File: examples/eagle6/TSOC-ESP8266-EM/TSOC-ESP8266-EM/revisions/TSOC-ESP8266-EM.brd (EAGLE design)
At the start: 38.1 x 25.4 mm, 21 parts, among them Q1 MMBT2222A, U1 ESP8266-12-12W

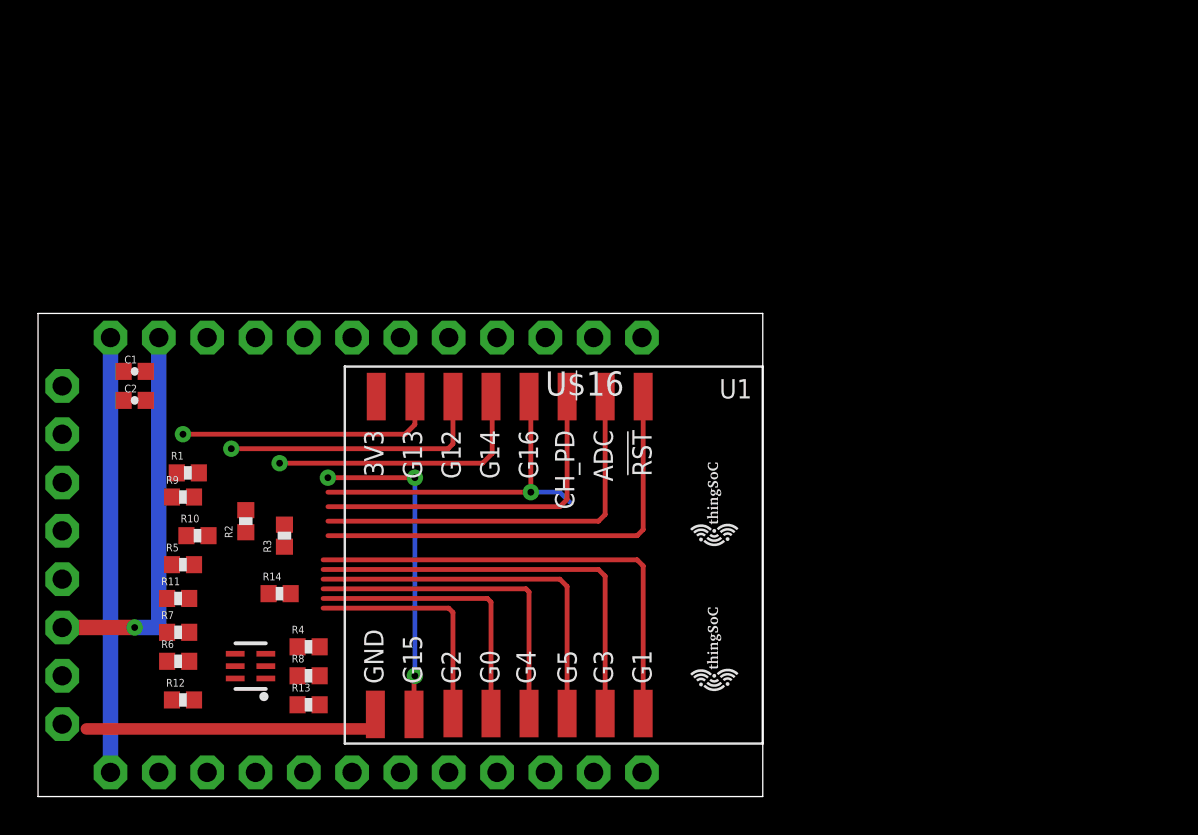
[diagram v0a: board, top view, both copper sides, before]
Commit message: update modules
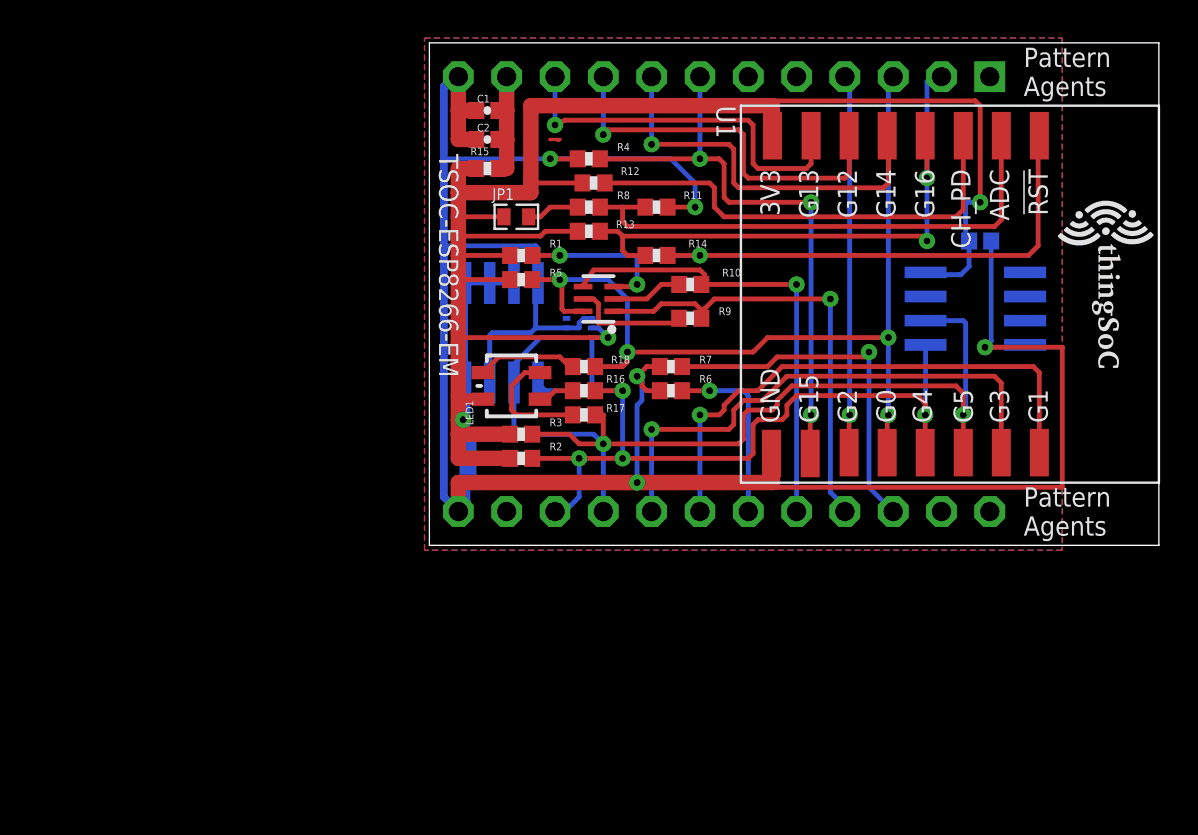
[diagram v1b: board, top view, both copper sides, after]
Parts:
- removed U$16: TSOC-32-BB, thingSoC:TSOC-BB-S32
- added C3, C4: 0.1uF, PatternAgents-ProtoPads:0402-CAP
- added JP1: (no value), PatternAgents-ProtoPads:JMP-2-NO-0402
- added LED1: LED-TRICOLOR, SparkFun-LED:LED-TRICOLOR-SMD
- added R15: 0.01, PatternAgents-ProtoPads:0402-RES
- added R16, R17, R18: 560, PatternAgents-ProtoPads:0402-RES
- added TSOC: TSOC-24-BB, thingSoC:TSOC-BB-S24
- added U$11: PA_LOGO_SYMMED, PatternAgents-Logos:PA_LOGO_AGENT_MED_SYM
- added U2: EEPROM-I2CSMD, SparkFun-DigitalIC:SO08
- added U3: TMP102, SparkFun-Sensors:SOT563
- added U4: ATECC108, SparkFun-DigitalIC:SOIC8
- U$19, U$20: value TSOC-LOGO-SMALL -> TSOC-LOGO-MED; device thingSoC:TSOC-LOGO-SML -> thingSoC:TSOC-LOGO-MED
- moved R12 34.7 mm to (8.89, 19.6), turned to 180 degrees
- moved R11 32.5 mm to (12.2, 18.3)
- moved U$20 31.1 mm to (35.8, 17.0), turned to 270 degrees
- moved R4 29.6 mm to (8.64, 20.8)
- moved R6 29.6 mm to (13.0, 8.64)
- moved R7 29.4 mm to (13.0, 9.91)
- moved R10 29.1 mm to (14.0, 14.2), turned to 180 degrees
- moved R13 28.9 mm to (8.64, 17.0), turned to 180 degrees
- moved R8 28.7 mm to (8.64, 18.3), turned to 180 degrees
- moved R9 28.3 mm to (14.0, 12.4), turned to 180 degrees
- moved R14 26.6 mm to (12.2, 15.7)
- moved Q1 26.6 mm to (9.14, 13.5)
- moved U1 24.9 mm to (27.2, 13.5)
- moved R5 23.3 mm to (5.08, 14.5), turned to 180 degrees
- moved C1 23.1 mm to (3.30, 23.4)
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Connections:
- net RESET renamed !RST
- removed net !DBG: U$16.1E
- removed net A0: R8.2, U$16.1C
- new net !DCD: TSOC.2C
- new net !RI: TSOC.1C
- new net 3V3I: C1.1, C2.1, R15.2, TSOC.11B
- new net ADC_RAW: JP1.2, R8.2
- new net BLU: LED1.B, R16.2
- new net GRN: LED1.G, R17.2
- new net RED: LED1.R, R18.2
- net !CTS: now also TSOC.6C; no longer U$16.6C, U$16.7E
- net !DSR: now also TSOC.3C; no longer U$16.3C
- net !DTR: now also TSOC.4C; no longer U$16.3E, U$16.4C
- net !RTS: now also TSOC.5C; no longer U$16.2E, U$16.5C
- net 3V3: now also C3.2, C4.2, JP1.1, LED1.A, R15.1, U2.1, U2.2, U2.3, U2.8, U3.5, U4.8; no longer C1.1, C2.1, U$16.11B, U$16.6E
- net GND: now also C3.1, C4.1, TSOC.12B, TSOC.12C, U2.4, U2.7, U3.2, U3.4, U4.4; no longer U$16.12B, U$16.12C, U$16.8E
- net GPIO0: now also R18.1, TSOC.3B
- net GPIO1: now also TSOC.7C; no longer U$16.4E, U$16.7C
- net GPIO12: now also TSOC.9B; no longer U$16.9B
- net GPIO13: now also TSOC.10B; no longer U$16.10B
- net GPIO14: now also TSOC.8B; no longer U$16.8B
- net GPIO15: now also TSOC.7B; no longer U$16.7B
- net GPIO16: now also TSOC.2B; no longer U$16.2C
- net GPIO2: now also TSOC.4B; no longer U$16.1B
- net GPIO3: now also TSOC.8C; no longer U$16.5E, U$16.8C
- net GPIO4: now also R16.1, TSOC.10C, U2.5, U3.6, U4.5; no longer U$16.10C
- net GPIO5: now also R17.1, TSOC.9C, U2.6, U3.1, U4.6; no longer U$16.9C
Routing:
- net GND: track 38.9 -> 132.4 mm, vias 0 -> 5
- net 3V3: track 20.3 -> 108.5 mm, vias 1 -> 3
- net GPIO5: track 19.7 -> 52.7 mm, vias 0 -> 2
- net GPIO0: track 14.8 -> 47.3 mm, vias 0 -> 4
- net GPIO4: track 17.3 -> 45.8 mm, vias 0 -> 4
- net !DTR: track 0.00 -> 24.6 mm, vias 0 -> 1
- net !RTS: track 0.00 -> 24.5 mm, vias 0 -> 1
- net !DSR: track 0.00 -> 19.1 mm, vias 0 -> 1
- net !RST: track 23.7 -> 37.3 mm, vias 0 -> 3
- net GPIO15: track 17.0 -> 30.6 mm
- net GPIO16: track 18.0 -> 31.1 mm, vias 1 -> 2
- net !CTS: track 0.00 -> 9.69 mm, vias 0 -> 1
- net GPIO2: track 12.2 -> 19.9 mm, vias 0 -> 1
- net ADC: track 20.9 -> 27.7 mm
- net GRN: track 0.00 -> 6.40 mm
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- added copper zone on layer 1, net GND
- added copper zone on layer 16, net GND
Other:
- board size 38.1 x 25.4 mm -> 38.4 x 26.4 mm
- board text added: "!CS"
- board text added: "!CTS"
- board text added: "!DSR"
- board text added: "!DTR"
- board text added: "3V3"
- board text added: "5V0"
- board text added: "GND"
- board text added: "IO1"
- board text added: "MISO"
- board text added: "MOSI"
- board text added: "NC"
- board text added: "Pattern Agents"
- board text added: "PatternAgents"
- board text added: "RTS"
- board text added: "RXD"
- board text added: "SCK"
- board text added: "SCL"
- board text added: "SDA"
- board text added: "SS1"
- board text added: "SS2"
- board text added: "TSOC-ESP8266-EM"
- board text added: "TXD"
- board text added: "U3"
